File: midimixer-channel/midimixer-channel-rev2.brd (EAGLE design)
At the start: 50.8 x 223.5 mm, 140 parts, among them IC1 74LS595D, IC2 74LS595D, IC3 74LS595D, IC4 74165D, IC5 74165D, T1 MMBT2222A, T2 MMBT2222A, U1 LM1117IMPX-3.3/NOPB

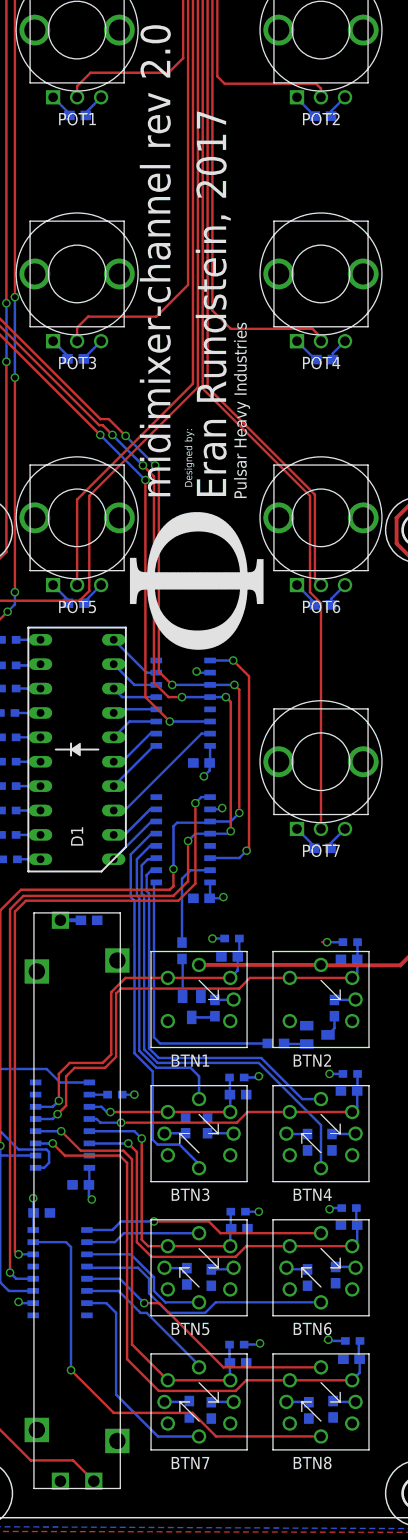
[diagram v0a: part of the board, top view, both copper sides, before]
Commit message: wip
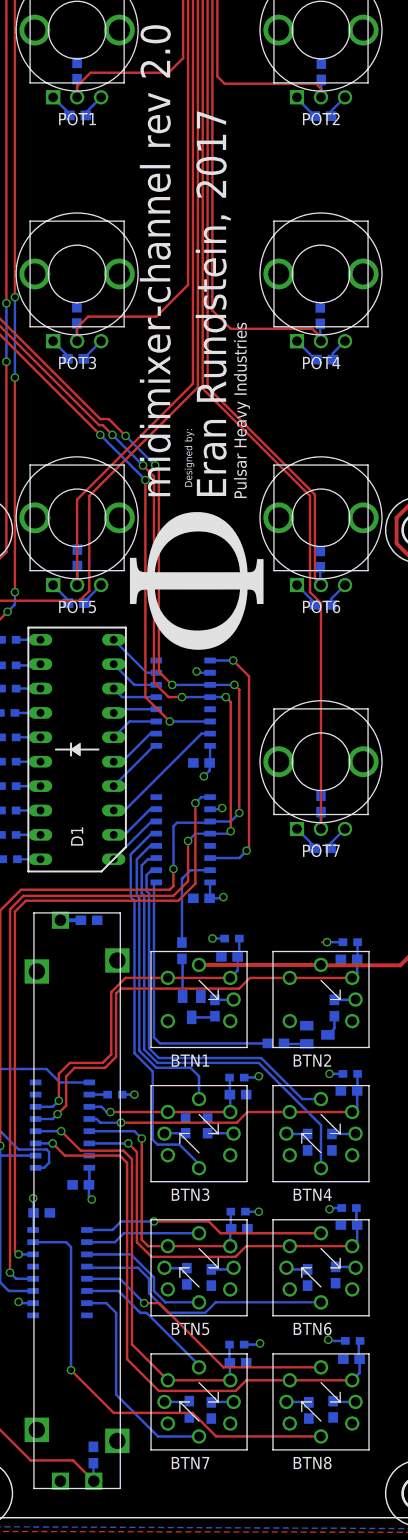
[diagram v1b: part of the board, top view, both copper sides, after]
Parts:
- added C42, C43, C44, C45, C46, C47, C48, C49: 0.01uF, microbuilder:0603
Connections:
- net FADER: now also C42.2
- net GND: now also C42.1, C43.1, C44.1, C45.1, C46.1, C47.1, C48.1, C49.1
- net POT1: now also C46.2
- net POT2: now also C49.2
- net POT3: now also C45.2
- net POT4: now also C48.2
- net POT5: now also C44.2
- net POT6: now also C47.2
- net POT7: now also C43.2
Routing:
- net POT5: track 101.4 -> 103.4 mm
- net POT3: track 86.8 -> 88.7 mm
- net POT6: track 100.9 -> 102.8 mm
- net FADER: track 212.5 -> 214.4 mm
- net POT1: track 62.9 -> 64.8 mm
- net POT4: track 84.8 -> 86.6 mm
- net POT2: track 55.3 -> 57.1 mm
- net POT7: track 126.8 -> 128.5 mm
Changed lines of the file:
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@@
 <layer number="24" name="bOrigins" color="15" fill="1" visible="yes" active="yes"/>
 <layer number="25" name="tNames" color="7" fill="1" visible="yes" active="yes"/>
-<layer number="26" name="bNames" color="7" fill="1" visible="no" active="yes"/>
+<layer number="26" name="bNames" color="7" fill="1" visible="yes" active="yes"/>
 <layer number="27" name="tValues" color="7" fill="1" visible="no" active="yes"/>
 <layer number="28" name="bValues" color="7" fill="1" visible="no" active="yes"/>
@@
 <element name="POT2" library="keves" package="PTV09A-4" value="" x="38.1" y="154.94"/>
 <element name="POT7" library="keves" package="PTV09A-4" value="" x="38.1" y="78.74"/>
-<element name="POT4" library="keves" package="PTV09A-4" value="" x="38.1" y="129.54"/>
+<element name="POT4" library="keves" package="PTV09A-4" value="" x="38.1" y="129.54" smashed="yes">
+<attribute name="NAME" x="36.068" y="119.634" size="1.27" layer="21"/>
+</element>
 <element name="POT5" library="keves" package="PTV09A-4" value="" x="12.7" y="104.14"/>
 <element name="POT6" library="keves" package="PTV09A-4" value="" x="38.1" y="104.14"/>
-<element name="POT3" library="keves" package="PTV09A-4" value="" x="12.7" y="129.54"/>
+<element name="POT3" library="keves" package="PTV09A-4" value="" x="12.7" y="129.54" smashed="yes">
+<attribute name="NAME" x="10.668" y="119.634" size="1.27" layer="21"/>
+</element>
 <element name="POT1" library="keves" package="PTV09A-4" value="" x="12.7" y="154.94"/>
 <element name="LCD" library="keves" package="SSD1306-7PIN-NO-HOLES" value="SSD1306-7PINWITHOUT-HOLES" x="25.4" y="195.58"/>
@@
 <element name="C39" library="microbuilder" package="0603" value="0.01uF" x="38.2524" y="69.723" rot="MR180"/>
 <element name="C40" library="microbuilder" package="0603" value="0.01uF" x="13.9446" y="62.23" rot="MR0"/>
+<element name="C42" library="microbuilder" package="0603" value="0.01uF" x="14.4018" y="6.5278" smashed="yes" rot="MR270">
+<attribute name="NAME" x="13.462" y="7.5692" size="0.8128" layer="26" font="vector" ratio="18" rot="MR270"/>
+<attribute name="VALUE" x="15.1638" y="4.7498" size="0.4064" layer="28" font="vector" ratio="10" rot="MR270"/>
+</element>
+<element name="C43" library="microbuilder" package="0603" value="0.01uF" x="38.1" y="74.3458" smashed="yes" rot="MR270">
+<attribute name="NAME" x="39.9796" y="75.311" size="0.8128" layer="26" font="vector" ratio="18" rot="MR270"/>
+<attribute name="VALUE" x="38.862" y="72.5678" size="0.4064" layer="28" font="vector" ratio="10" rot="MR270"/>
+</element>
+<element name="C44" library="microbuilder" package="0603" value="0.01uF" x="12.7254" y="99.9744" smashed="yes" rot="MR270">
+<attribute name="NAME" x="14.5542" y="101.0158" size="0.8128" layer="26" font="vector" ratio="18" rot="MR270"/>
+<attribute name="VALUE" x="13.4874" y="98.1964" size="0.4064" layer="28" font="vector" ratio="10" rot="MR270"/>
+</element>
+<element name="C45" library="microbuilder" package="0603" value="0.01uF" x="12.6746" y="125.222" smashed="yes" rot="MR270">
+<attribute name="NAME" x="14.5288" y="125.8316" size="0.8128" layer="26" font="vector" ratio="18" rot="MR270"/>
+<attribute name="VALUE" x="13.4366" y="123.444" size="0.4064" layer="28" font="vector" ratio="10" rot="MR270"/>
+</element>
+<element name="C46" library="microbuilder" package="0603" value="0.01uF" x="12.7" y="150.6728" smashed="yes" rot="MR270">
+<attribute name="NAME" x="14.5288" y="151.3586" size="0.8128" layer="26" font="vector" ratio="18" rot="MR270"/>
+<attribute name="VALUE" x="13.462" y="148.8948" size="0.4064" layer="28" font="vector" ratio="10" rot="MR270"/>
+</element>
+<element name="C47" library="microbuilder" package="0603" value="0.01uF" x="38.0238" y="99.8474" smashed="yes" rot="MR270">
+<attribute name="NAME" x="39.7764" y="100.4062" size="0.8128" layer="26" font="vector" ratio="18" rot="MR270"/>
+<attribute name="VALUE" x="38.7858" y="98.0694" size="0.4064" layer="28" font="vector" ratio="10" rot="MR270"/>
+</element>
+<element name="C48" library="microbuilder" package="0603" value="0.01uF" x="38.0238" y="125.1966" smashed="yes" rot="MR270">
+<attribute name="NAME" x="39.8018" y="125.7808" size="0.8128" layer="26" font="vector" ratio="18" rot="MR270"/>
+<attribute name="VALUE" x="38.7858" y="123.4186" size="0.4064" layer="28" font="vector" ratio="10" rot="MR270"/>
+</element>
+<element name="C49" library="microbuilder" package="0603" value="0.01uF" x="38.1254" y="150.5966" smashed="yes" rot="MR270">
+<attribute name="NAME" x="39.9288" y="151.3586" size="0.8128" layer="26" font="vector" ratio="18" rot="MR270"/>
+<attribute name="VALUE" x="38.8874" y="148.8186" size="0.4064" layer="28" font="vector" ratio="10" rot="MR270"/>
+</element>
 </elements>
 <signals>
@@
 <wire x1="35.6616" y1="147.955" x2="35.6616" y2="147.7654" width="0.254" layer="16"/>
 <wire x1="35.6616" y1="147.7654" x2="37.4532" y2="145.9738" width="0.254" layer="16"/>
+<contactref element="C42" pad="1"/>
+<contactref element="C43" pad="1"/>
+<contactref element="C44" pad="1"/>
+<contactref element="C45" pad="1"/>
+<contactref element="C46" pad="1"/>
+<contactref element="C47" pad="1"/>
+<contactref element="C48" pad="1"/>
+<contactref element="C49" pad="1"/>
 </signal>
 <signal name="NRST">
@@
 <wire x1="27.813" y1="191.516" x2="27.305" y2="191.008" width="0.254" layer="1"/>
 <wire x1="27.305" y1="191.008" x2="27.305" y2="150.114" width="0.254" layer="1"/>
+<contactref element="C49" pad="2"/>
+<wire x1="38.1254" y1="149.7466" x2="38.1254" y2="148.6916" width="0.254" layer="16"/>
+<wire x1="38.1254" y1="148.6916" x2="38.1" y2="148.6662" width="0.254" layer="16"/>
+<wire x1="38.1" y1="148.6662" x2="38.1" y2="147.94" width="0.254" layer="16"/>
 </signal>
 <signal name="N$11">
@@
 <wire x1="1.524" y1="42.418" x2="2.032" y2="41.91" width="0.254" layer="1"/>
 <wire x1="2.032" y1="41.91" x2="2.032" y2="11.811" width="0.254" layer="1"/>
+<contactref element="C42" pad="2"/>
+<wire x1="14.4018" y1="5.6778" x2="14.4018" y2="3.8481" width="0.254" layer="16"/>
+<wire x1="14.4018" y1="3.8481" x2="14.4399" y2="3.81" width="0.254" layer="16"/>
 </signal>
 <signal name="POT4">
@@
 <wire x1="27.492" y1="194.878" x2="27.051" y2="194.437" width="0.254" layer="16"/>
 <via x="27.051" y="194.437" extent="1-16" drill="0.6"/>
+<contactref element="C48" pad="2"/>
+<wire x1="38.0238" y1="124.3466" x2="38.0238" y2="122.6162" width="0.254" layer="16"/>
+<wire x1="38.0238" y1="122.6162" x2="38.1" y2="122.54" width="0.254" layer="16"/>
 </signal>
 <signal name="POT6">
@@
 <wire x1="26.162" y1="186.436" x2="26.035" y2="186.309" width="0.254" layer="16"/>
 <wire x1="26.289" y1="186.055" x2="26.035" y2="186.309" width="0.254" layer="1"/>
+<contactref element="C47" pad="2"/>
+<wire x1="38.0238" y1="98.9974" x2="38.0238" y2="97.2162" width="0.254" layer="16"/>
+<wire x1="38.0238" y1="97.2162" x2="38.1" y2="97.14" width="0.254" layer="16"/>
 </signal>
 <signal name="POT1">
@@
 <wire x1="23.114" y1="181.483" x2="23.749" y2="180.848" width="0.254" layer="1"/>
 <wire x1="23.749" y1="180.848" x2="23.749" y2="152.019" width="0.254" layer="1"/>
+<contactref element="C46" pad="2"/>
+<wire x1="12.7" y1="149.8228" x2="12.7" y2="147.94" width="0.254" layer="16"/>
 </signal>
 <signal name="POT3">
 <contactref element="POT3" pad="CENTER"/>
-<wire x1="12.7" y1="122.54" x2="12.7" y2="123.952" width="0.254" layer="1"/>
+<wire x1="12.7" y1="122.54" x2="12.7" y2="122.555" width="0.254" layer="1"/>
 <wire x1="12.7" y1="123.952" x2="13.843" y2="125.095" width="0.254" layer="1"/>
 <wire x1="13.843" y1="125.095" x2="20.955" y2="125.095" width="0.254" layer="1"/>
@@
 <via x="26.035" y="194.945" extent="1-16" drill="0.6"/>
 <wire x1="26.035" y1="194.945" x2="26.035" y2="187.706" width="0.254" layer="1"/>
+<contactref element="C45" pad="2"/>
+<wire x1="12.7" y1="123.952" x2="12.7" y2="122.555" width="0.254" layer="1"/>
+<wire x1="12.7" y1="122.555" x2="12.6746" y2="122.5296" width="0.254" layer="1"/>
+<wire x1="12.6746" y1="122.5296" x2="12.6492" y2="122.5296" width="0.254" layer="1"/>
+<wire x1="12.6746" y1="124.372" x2="12.6746" y2="122.5654" width="0.254" layer="16"/>
+<wire x1="12.6746" y1="122.5654" x2="12.7" y2="122.54" width="0.254" layer="16"/>
 </signal>
 <signal name="POT5">
@@
 <wire x1="25.007" y1="191.758" x2="24.638" y2="191.389" width="0.254" layer="16"/>
 <wire x1="24.638" y1="191.389" x2="24.638" y2="187.96" width="0.254" layer="16"/>
+<contactref element="C44" pad="2"/>
+<wire x1="12.7254" y1="99.1244" x2="12.7254" y2="97.1654" width="0.254" layer="16"/>
+<wire x1="12.7254" y1="97.1654" x2="12.7" y2="97.14" width="0.254" layer="16"/>
 </signal>
 <signal name="POT7">
@@
 <wire x1="25.273" y1="186.944" x2="25.273" y2="185.293" width="0.254" layer="16"/>
 <wire x1="25.273" y1="185.293" x2="25.527" y2="185.039" width="0.254" layer="16"/>
+<contactref element="C43" pad="2"/>
+<wire x1="38.1" y1="73.4958" x2="38.1" y2="71.74" width="0.254" layer="16"/>
 </signal>
 <signal name="LCD_MISO_UNUSED">
